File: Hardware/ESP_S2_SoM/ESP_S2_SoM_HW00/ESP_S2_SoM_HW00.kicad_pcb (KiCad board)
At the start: 6 copper layers, 26.3 x 23.2 mm, 58 parts, among them J101 DF40C-60DP-0.4V(51), J102 Bare PCB USB C, SW401 SW_Push, SW402 SW_Push, U201 BQ24075RGTR, U301 MIC5528-3.3YMT-T5, U401 ESP32-S2FH4, Y601 Crystal_GND24_Small

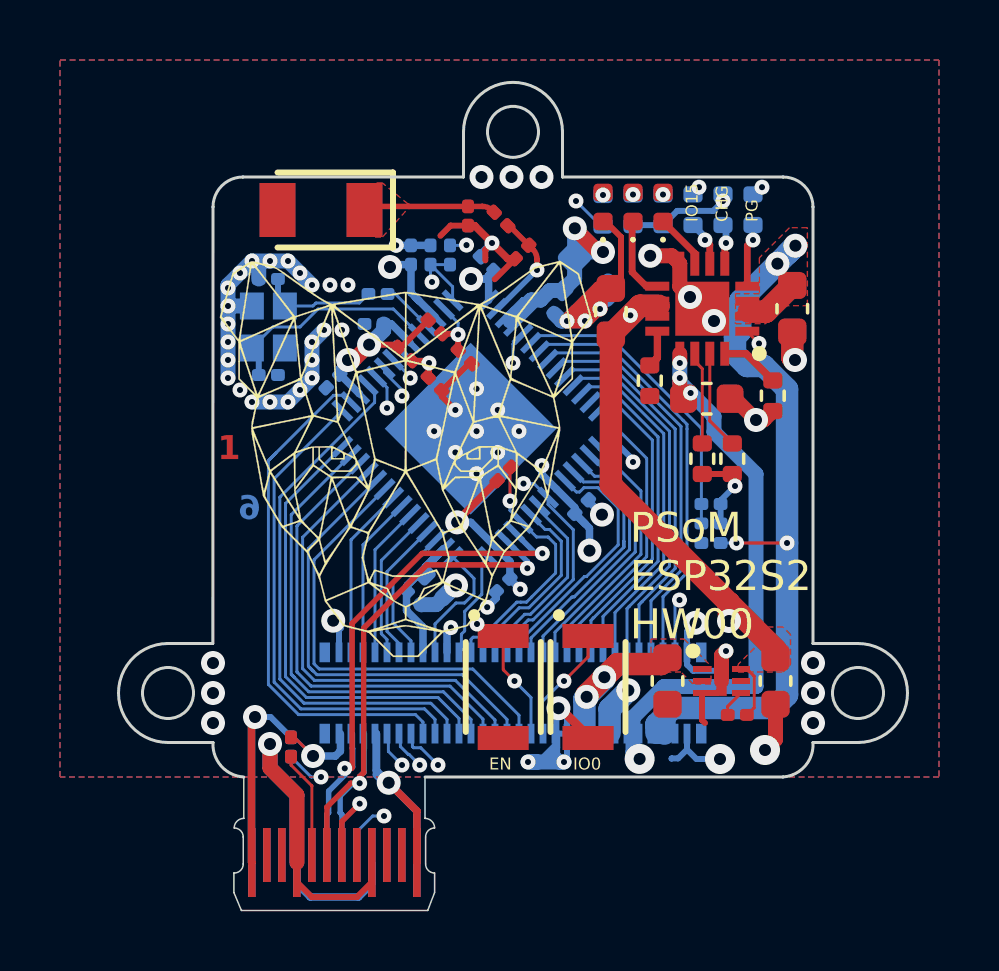
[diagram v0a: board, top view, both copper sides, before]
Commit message: final esp32s2 update?
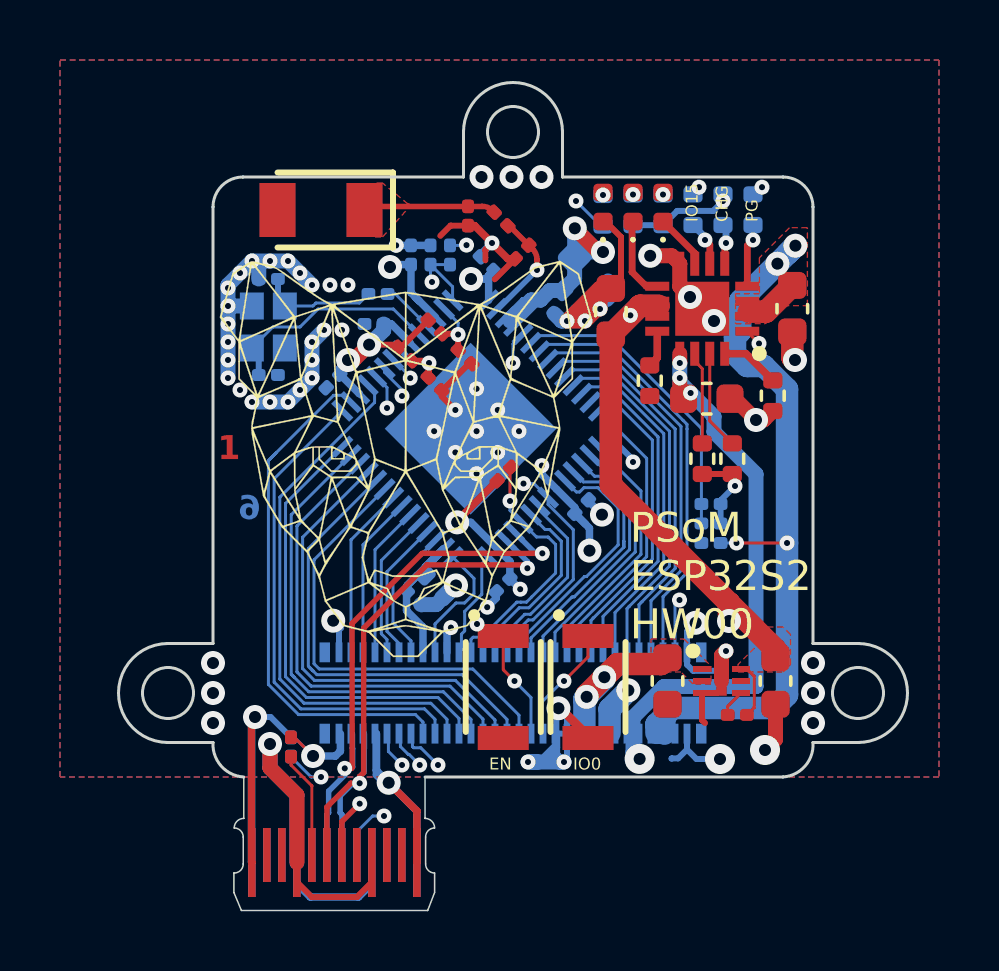
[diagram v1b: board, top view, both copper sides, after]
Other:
- outline, holes or cut-outs redrawn
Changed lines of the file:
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@@
     )
   )
-  (gr_circle (center 124.05 106.25) (end 125.7 106.25)
+  (gr_circle (center 124.5 106.2) (end 126.15 106.2)
     (stroke (width 0.15) (type solid)) (fill solid) (layer "B.Mask"))
-  (gr_circle (center 136.05 87) (end 137.7 87)
+  (gr_circle (center 136 87.5) (end 137.65 87.5)
     (stroke (width 0.15) (type solid)) (fill solid) (layer "B.Mask"))
-  (gr_circle (center 148 106.25) (end 149.65 106.25)
+  (gr_circle (center 147.5 106.2) (end 149.15 106.2)
     (stroke (width 0.15) (type solid)) (fill solid) (layer "B.Mask"))
-  (gr_circle (center 136.05 87) (end 137.7 87)
+  (gr_circle (center 136 87.5) (end 137.65 87.5)
     (stroke (width 0.15) (type solid)) (fill solid) (layer "F.Mask"))
-  (gr_circle (center 136.05 87) (end 137.7 87)
+  (gr_circle (center 124.5 106.2) (end 126.15 106.2)
     (stroke (width 0.15) (type solid)) (fill solid) (layer "F.Mask"))
-  (gr_circle (center 124.05 106.25) (end 125.7 106.25)
-    (stroke (width 0.15) (type solid)) (fill solid) (layer "F.Mask"))
-  (gr_circle (center 148 106.25) (end 149.65 106.25)
+  (gr_circle (center 147.5 106.2) (end 149.15 106.2)
     (stroke (width 0.15) (type solid)) (fill solid) (layer "F.Mask"))
   (gr_line (start 145 89) (end 137.65 89)
     (stroke (width 0.1) (type default)) (layer "Edge.Cuts"))
-  (gr_line (start 124.5 104.54997) (end 125.994988 104.55)
+  (gr_line (start 124.5 104.55) (end 126 104.55)
     (stroke (width 0.1) (type default)) (layer "Edge.Cuts"))
   (gr_arc (start 145 89) (mid 145.707106 89.292893) (end 146 90)
     (stroke (width 0.1) (type default)) (layer "Edge.Cuts"))
-  (gr_arc (start 134.35 87.505012) (mid 135.995 85.844964) (end 137.650031 87.495012)
+  (gr_arc (start 134.35 87.5) (mid 136 85.85) (end 137.65 87.5)
     (stroke (width 0.1) (type default)) (layer "Edge.Cuts"))
-  (gr_arc (start 124.51 107.85) (mid 122.849954 106.205) (end 124.5 104.54997)
+  (gr_arc (start 124.5 107.85) (mid 122.85 106.2) (end 124.5 104.55)
     (stroke (width 0.1) (type default)) (layer "Edge.Cuts"))
-  (gr_arc (start 146 107.849985) (mid 145.738176 108.632099) (end 145 109)
+  (gr_arc (start 146 107.85) (mid 145.738173 108.632107) (end 145 109)
     (stroke (width 0.1) (type default)) (layer "Edge.Cuts"))
-  (gr_circle (center 124.5 106.2) (end 123.65 106.2)
+  (gr_circle (center 124.5 106.2) (end 125.35 106.2)
     (stroke (width 0.1) (type default)) (fill none) (layer "Edge.Cuts"))
-  (gr_line (start 147.489976 104.549985) (end 146 104.549985)
+  (gr_line (start 147.5 104.55) (end 146 104.55)
     (stroke (width 0.1) (type default)) (layer "Edge.Cuts"))
   (gr_line (start 134.35 89) (end 127 89)
     (stroke (width 0.1) (type default)) (layer "Edge.Cuts"))
-  (gr_circle (center 147.499977 106.199985) (end 148.349977 106.199985)
+  (gr_circle (center 147.5 106.2) (end 148.35 106.2)
     (stroke (width 0.1) (type default)) (fill none) (layer "Edge.Cuts"))
-  (gr_line (start 146 90) (end 146 104.549985)
+  (gr_line (start 146 90) (end 146 104.55)
     (stroke (width 0.1) (type default)) (layer "Edge.Cuts"))
-  (gr_line (start 125.994988 104.55) (end 126 90)
+  (gr_line (start 126 104.55) (end 126 90)
     (stroke (width 0.1) (type default)) (layer "Edge.Cuts"))
-  (gr_line (start 134.35 87.505012) (end 134.35 89)
+  (gr_line (start 134.35 87.5) (end 134.35 89)
     (stroke (width 0.1) (type default)) (layer "Edge.Cuts"))
-  (gr_line (start 146 107.849985) (end 147.499977 107.850015)
+  (gr_line (start 146 107.85) (end 147.5 107.85)
     (stroke (width 0.1) (type default)) (layer "Edge.Cuts"))
-  (gr_circle (center 136.000002 87.495012) (end 136.000001 86.645012)
+  (gr_circle (center 136 87.5) (end 136.85 87.5)
     (stroke (width 0.1) (type default)) (fill none) (layer "Edge.Cuts"))
   (gr_arc (start 127.026853 109) (mid 126.275244 108.637676) (end 126 107.85)
@@
   (gr_line (start 145 109) (end 133.066853 109)
     (stroke (width 0.1) (type default)) (layer "Edge.Cuts"))
-  (gr_line (start 137.650031 87.495012) (end 137.65 89)
+  (gr_line (start 137.65 87.5) (end 137.65 89)
     (stroke (width 0.1) (type default)) (layer "Edge.Cuts"))
   (gr_arc (start 126 90) (mid 126.292893 89.292894) (end 127 89)
     (stroke (width 0.1) (type default)) (layer "Edge.Cuts"))
-  (gr_line (start 124.51 107.85) (end 126 107.85)
+  (gr_line (start 124.5 107.85) (end 126 107.85)
     (stroke (width 0.1) (type default)) (layer "Edge.Cuts"))
-  (gr_arc (start 147.489976 104.549985) (mid 149.150023 106.194984) (end 147.499977 107.850015)
+  (gr_arc (start 147.5 104.55) (mid 149.15 106.2) (end 147.5 107.85)
     (stroke (width 0.1) (type default)) (layer "Edge.Cuts"))
   (gr_text "1" (at 126.15 98.5) (layer "F.Cu")
